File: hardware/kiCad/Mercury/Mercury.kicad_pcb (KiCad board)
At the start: 4 copper layers, 100 x 80 mm, 120 parts, among them J1 SWD, J10 OUTPUT, J11 Analog I/O, J12 Power Rails, J13 5-1814832-1, J14 5-1814832-1, J2 UART1, J3 I2C2, J4 UART1, J5 SPI1, J6 SPI2, J7 1981568-1, J8 Battery Input, J9 INPUT, Q1 AO3401A, SW1 SW_SPDT, U1 STM32F407VGT6, U2 AMS1117-3.3, U3 AMS1117-5.0, U4 MPU-6050, U5 W25N01GVZEIG_TR, U6 LPS25HB, U7 CC2500, U8 CC2592RGVR, U9 MAX-8Q, Y1 HSE 16MHz, Y2 26 MHz Oscillator

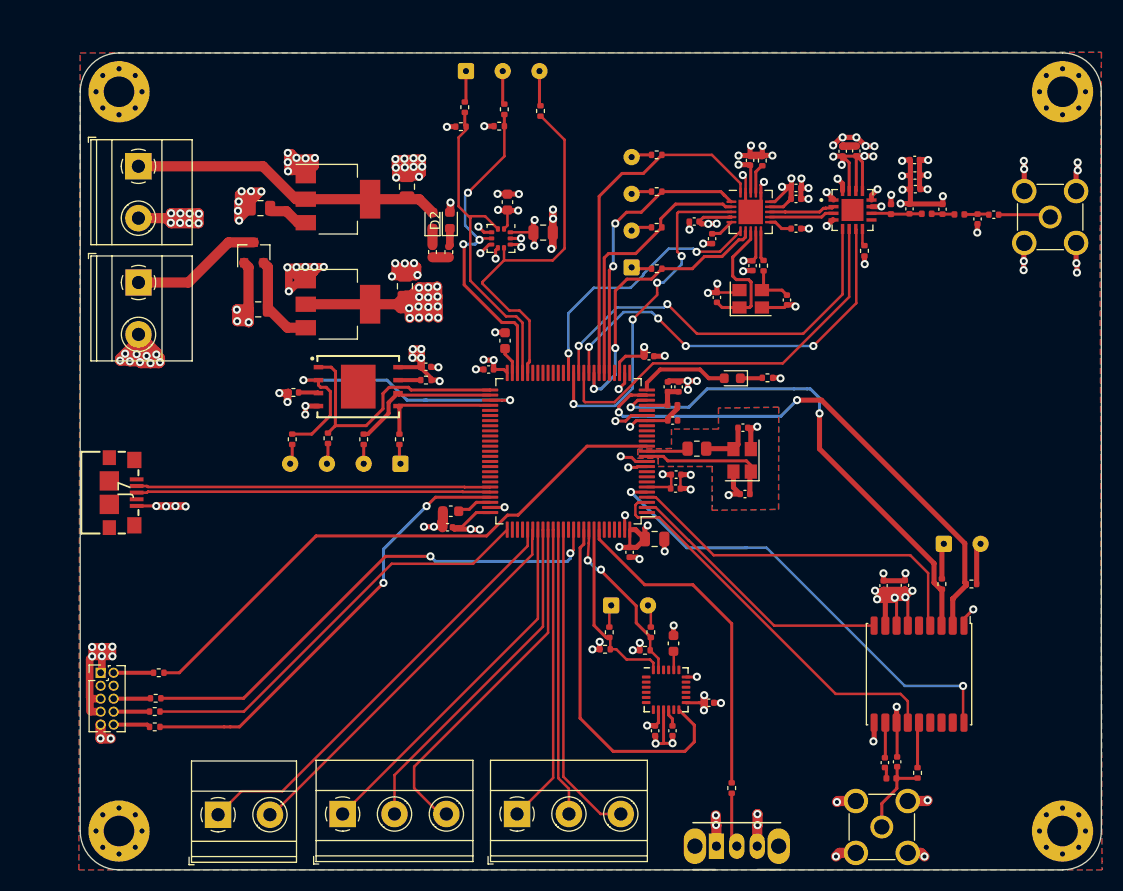
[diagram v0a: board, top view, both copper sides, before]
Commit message: Sent For Manufacture
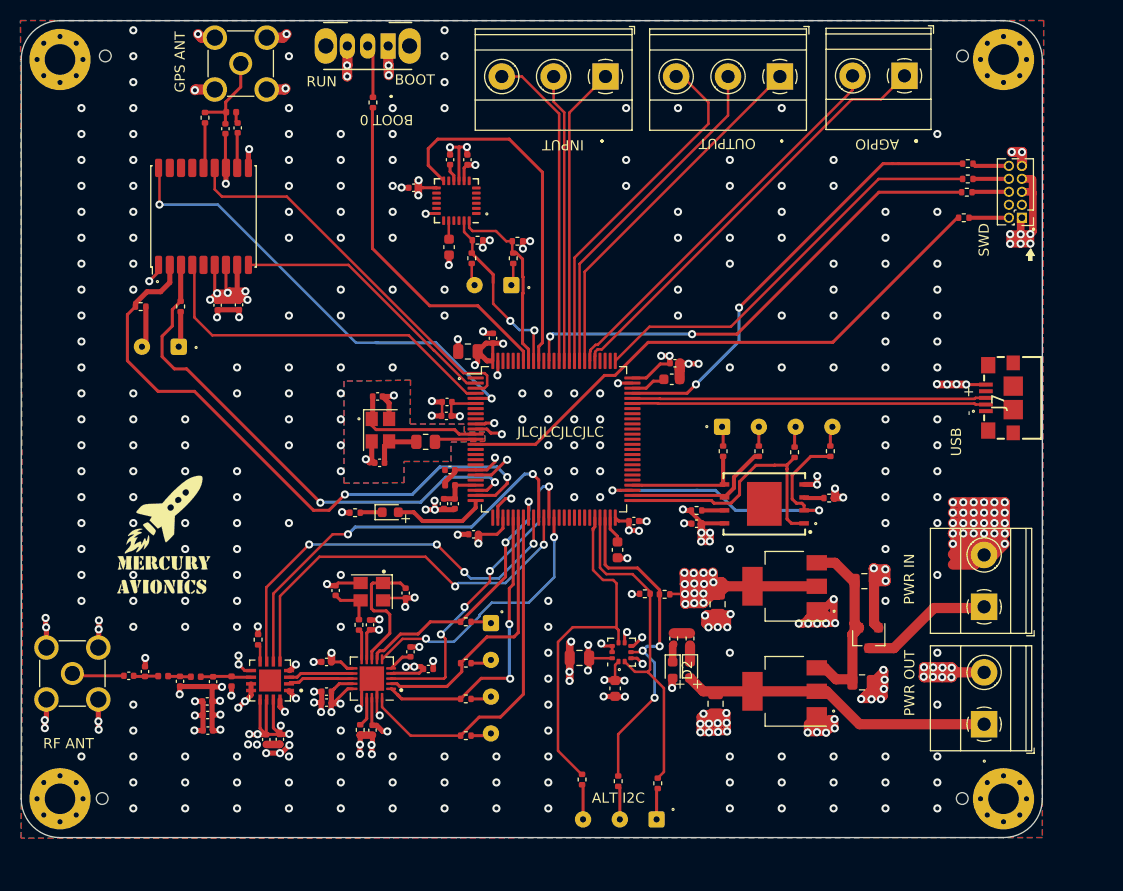
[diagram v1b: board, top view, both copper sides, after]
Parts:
- added G1: LOGO, LOGO:LOGO, F.Cu at (28.2, 67.1)
- moved H3 123.9 mm to (18.2, 20.6), turned to 180 degrees
- moved H2 120.1 mm to (18.2, 93.0), turned to 180 degrees
- moved H4 114.9 mm to (110.6, 20.6), turned to 180 degrees
- moved H1 110.9 mm to (110.6, 93.0), turned to 180 degrees
- moved J14 105.7 mm to (19.4, 80.8), turned to 0 degrees
- moved J1 100.6 mm to (112.4, 36.1), turned to 180 degrees
- moved J12 99.2 mm to (108.7, 85.7), turned to 90 degrees
- moved J11 98.8 mm to (100.9, 22.2), turned to 180 degrees
- moved J13 97.6 mm to (35.9, 21.0), turned to 180 degrees
- moved R10 96.9 mm to (107.1, 30.8), turned to 180 degrees
- moved C44 96.0 mm to (25.0, 81.0), turned to 0 degrees
- moved R11 95.2 mm to (107.1, 32.3), turned to 180 degrees
- moved R37 94.8 mm to (32.4, 26.3), turned to 90 degrees
- moved J7 94.5 mm to (114.3, 53.8), turned to 90 degrees
- moved R12 93.6 mm to (107.0, 33.6), turned to 180 degrees
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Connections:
- U6 pad 6: GND -> +3V3
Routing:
- net GND: track 292.4 -> 356.9 mm, vias 145 -> 380
- net UART1_RX: track 54.0 -> 62.4 mm
- net Vin: track 13.0 -> 19.7 mm
- net +3V3: track 183.0 -> 185.8 mm, vias 76 -> 77
- net UART1_TX: track 48.8 -> 51.7 mm
- net RF_GPO1: track 34.7 -> 32.0 mm
- net RF_CS: track 28.9 -> 27.0 mm
- net RF_LNA_EN: track 39.7 -> 41.4 mm, vias 0 -> 2
- net I2C1_SCL: track 16.8 -> 18.3 mm
- net ALT_INT_1: track 36.1 -> 34.6 mm
- net I2C2_SDA: track 32.9 -> 34.2 mm
- net SPI1_SCK: track 28.2 -> 29.2 mm
- net I2C1_SDA: track 17.2 -> 18.1 mm
- net BOOT0: track 32.9 -> 33.7 mm
- net I2C2_SCL: track 32.5 -> 33.0 mm
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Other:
- outline, holes or cut-outs redrawn
- board text added: "+"
- board text added: "+3.3V"
- board text added: "+5V"
- board text added: "-"
- board text added: "AGPIO"
- board text added: "AGPIO1"
- board text added: "AGPIO2"
- board text added: "ALT"
- board text added: "ALT I2C"
- board text added: "BOOT"
- board text added: "BOOT 0"
- board text added: "CS"
- board text added: "Designed By Mois & Vik in 2021"
- board text added: "GND"
- board text added: "GPS ANT"
- board text added: "I1"
- board text added: "I2"
- board text added: "I3"
- board text added: "INPUT"
- board text added: "JLCJLCJLCJLC"
- board text added: "MISO"
- board text added: "MOSI"
- board text added: "Mercury Avionics Package"
- board text added: "O1"
- board text added: "O2"
- board text added: "O3"
- board text added: "OUTPUT"
- board text added: "PWR IN"
- board text added: "PWR OUT"
- board text added: "RF ANT"
- board text added: "RUN"
- board text added: "RX"
- board text added: "SCK"
- board text added: "SCL"
- board text added: "SDA"
- board text added: "SWD"
- board text added: "TX"
- board text added: "USB"
- board text added: "V1.0"
- board text added: "VIN"
